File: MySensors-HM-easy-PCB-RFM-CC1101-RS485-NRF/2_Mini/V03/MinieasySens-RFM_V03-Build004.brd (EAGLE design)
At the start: 63 x 33 mm, 39 parts, among them IC1 ATSHA204A, IC2 REG1117, IC3 LD117ADT50TR, IC4 LM1117MPX-ADJ, M1 ARDUINO-PRO-MINI-3.3V#NP, X1 1751264, X4 1751264

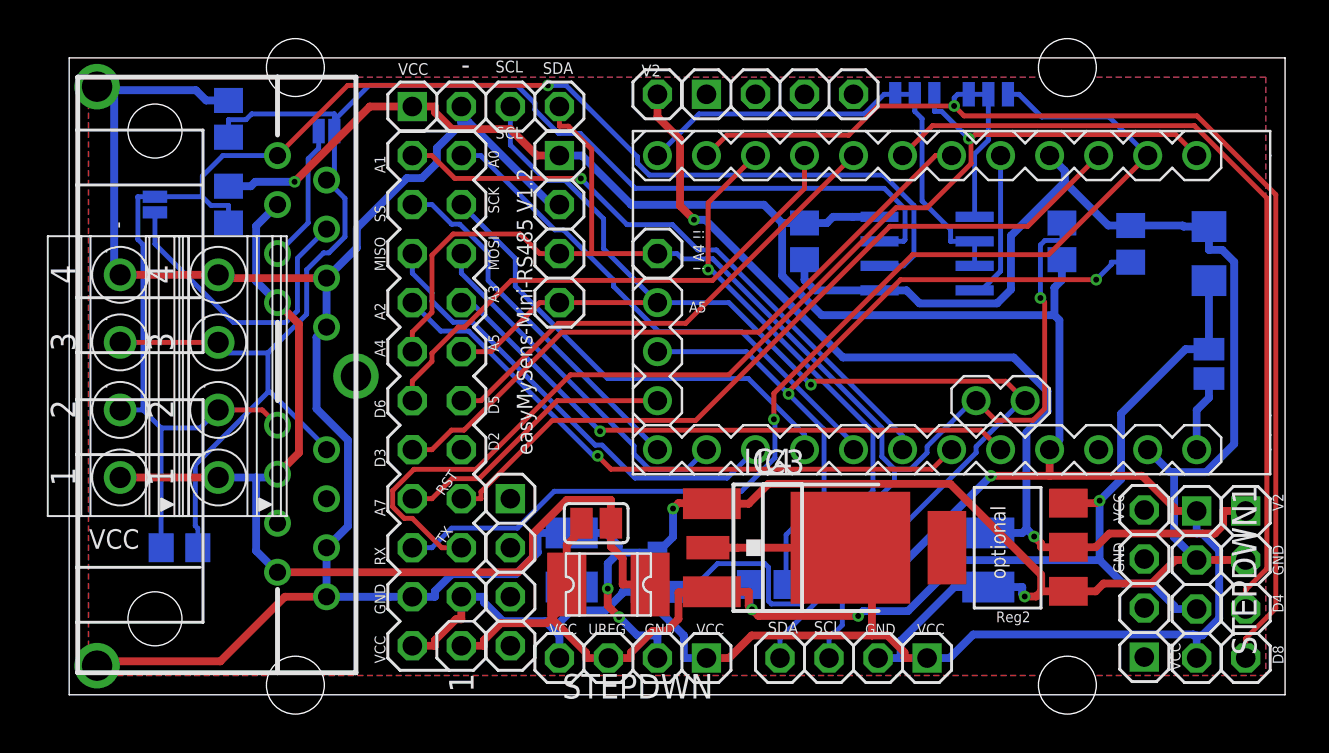
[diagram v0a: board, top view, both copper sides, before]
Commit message: Mini RFM-V03
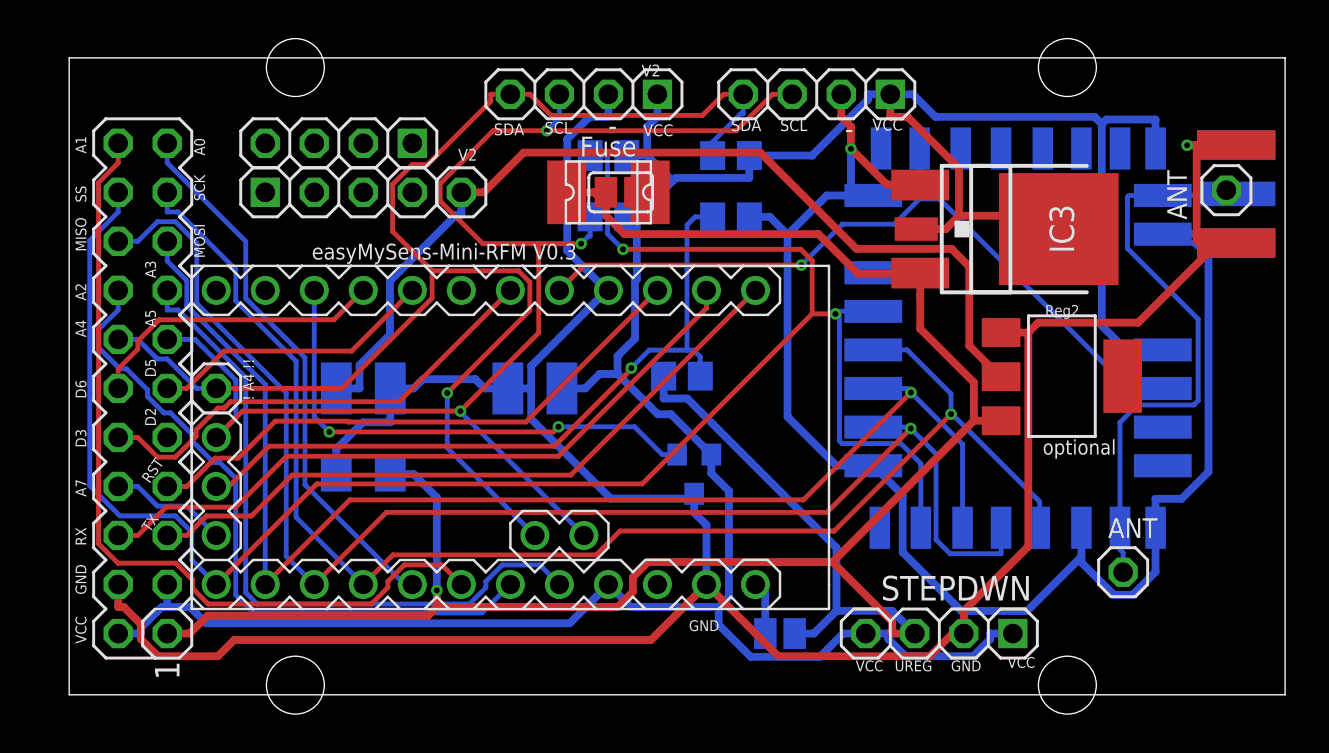
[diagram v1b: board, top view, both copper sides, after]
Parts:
- removed C10: 22p, rcl:C0805
- removed I2C-2, JP4, STEPDWN1, V2-: (no value), pinhead-2:1X04-S
- removed J2: (no value), RJ45:RJ45_2X_NARROW_SHILDPINS_NOCASE
- removed LAN1, LAN2: JUMPER-SMT_2_NC_PASTE_SILK, SparkFun-Jumpers:SMT-JUMPER_2_NC_PASTE_SILK
- removed R5: 150R, rcl:R0805
- removed R6, R8: 330R, rcl:R0805
- removed RS485: MAX487ECSA+, Maxim_By_element14_Batch_1:SOIC127P600X175-8N
- removed RX_SEL, TX_SEL: JUMPER-SMT_3_1-NC_TRACE_SILK, SparkFun-Jumpers:SMT-JUMPER_3_1-NC_TRACE_SILK
- removed X1, X4: 1751264, con-phoenix-350:1751264
- added ANT1, ANT2: (no value), pinhead:1X01
- added R4: 10k, rcl:M0805
- added RFM69W: RFM69HW, hoperf:RFM
- added U1: RFM69HCW, doug:RFM69HCW-XXXS2
- added X2: (no value), adafruit:SMA_EDGELAUNCH
- moved C6 45.3 mm to (15.2, 11.4), turned to 0 degrees
- moved C1 33.6 mm to (15.2, 15.9), turned to 180 degrees
- moved I2C-1 32.4 mm to (26.7, 31.1)
- moved RAW 26.3 mm to (36.8, 3.17), turned to 180 degrees
- moved A4 23.9 mm to (7.62, 15.9)
- moved M1 23.9 mm to (22.9, 13.3)
- moved R7 23.6 mm to (27.9, 24.8)
- moved JP2 23.0 mm to (14.0, 28.6), turned to 180 degrees
- moved JP1 21.6 mm to (14.0, 26.0), turned to 0 degrees
- moved R2 20.8 mm to (34.3, 24.8), turned to 0 degrees
- moved F1 20.3 mm to (27.9, 26.0)
- moved IC3 19.7 mm to (48.9, 24.1)
- moved IC4 19.7 mm to (47.0, 24.1)
- moved R3 17.7 mm to (34.3, 27.9), turned to 0 degrees
- moved RAW1 17.2 mm to (28.6, 26.0)
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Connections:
- removed net 4: J2.1-4, LAN1.1
- removed net 5: J2.1-5, LAN2.1
- removed net A: J2.1-1, J2.2-1, LAN1.2, R5.1, R6.2, RS485.6, X1.2, X4.2
- removed net B: J2.1-2, J2.2-2, LAN2.2, R5.2, R8.1, RS485.7, X1.3, X4.3
- removed net RX: RS485.1, RX_SEL.2
- removed net TX: RS485.2, RS485.3, TX_SEL.2
- new net ANT: ANT1.1, ANT2.1, RFM69W.ANT, U1.ANT, X2.P
- new net N$14: U1.DIO2
- new net N$15: U1.DIO1
- new net N$3: U1.RESET
- net A4: no longer I2C-2.3
- net A5: no longer I2C-2.4
- net D10_SS: now also R4.1, RFM69W.NSS, U1.NSS
- net D11_MOSI: now also RFM69W.MOSI, U1.MOSI
- net D12_MISO: now also RFM69W.MISO, U1.MISO
- net D13_SCK: now also RFM69W.SCK, U1.SCK
- net D2_INT0: now also RFM69W.DIO0, U1.DIO0; no longer RS485.4
- net D4: no longer V2-.3
- net D8: no longer RX_SEL.3, V2-.4
- net D9: no longer TX_SEL.3
- net GND: now also RFM69W.GNDA, RFM69W.GNDB, U1.GND_1, U1.GND_2, U1.GND_3, X2.GND@1, X2.GND@2, X2.GND@3, X2.GND@4; no longer C10.1, I2C-2.2, J2.1-6, J2.1-8, J2.2-6, J2.2-8, J2.G1, J2.G3, R8.2, RS485.5, STEPDWN1.2, V2-.2, X1.4, X4.4
- net RX0: no longer RX_SEL.1
- net TX1: no longer TX_SEL.1
- net UREG: no longer STEPDWN1.3
- net V2: no longer V2-.1
- net VCC: now also R4.2, RFM69W.VCC, U1.3.3V; no longer C10.2, I2C-2.1, R6.1, RS485.8, STEPDWN1.1, STEPDWN1.4
- net VIN: no longer J2.1-3, J2.1-7, J2.2-3, J2.2-7, X1.1, X4.1
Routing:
- net B: track 81.3 -> 0.00 mm
- net D10_SS: track 18.8 -> 98.8 mm, vias 0 -> 2
- net A: track 79.7 -> 0.00 mm, vias 1 -> 0
- net D8: track 58.4 -> 0.00 mm, vias 1 -> 0
- net VIN: track 55.0 -> 0.76 mm
- net D11_MOSI: track 18.6 -> 67.6 mm, vias 0 -> 1
- net D12_MISO: track 24.0 -> 72.7 mm, vias 0 -> 1
- net D13_SCK: track 24.3 -> 72.8 mm, vias 0 -> 1
- net UREG: track 71.7 -> 116.6 mm, vias 3 -> 1
- net D4: track 42.8 -> 0.00 mm
- net D2_INT0: track 7.75 -> 39.9 mm, vias 0 -> 1
- net ANT: track 0.00 -> 30.3 mm
- net TX1: track 59.2 -> 35.7 mm, vias 1 -> 0
- net RX0: track 57.1 -> 36.3 mm, vias 1 -> 0
- net GND: track 204.9 -> 223.7 mm, vias 4 -> 2
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- removed copper zone on layer 1, net GND
- removed copper zone on layer 16, net GND
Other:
- board text added: "ANT"
- board text added: "C4"
- board text added: "Fuse"
- board text added: "IN"
- board text added: "R4"
- board text added: "easyMySens-Mini-RFM V0.3"
- board text added: "easyMySens-RFM V0.3"
- board text removed: "+"
- board text removed: "120"
- board text removed: "Bus Pull"
- board text removed: "Bus Terminat."
- board text removed: "C10"
- board text removed: "D4"
- board text removed: "D8"
- board text removed: "Serial"
- board text removed: "easyMySens-Mini-RS485 V1.2"
- board text removed: "easyMySens-RS485-Mini V1.2"
